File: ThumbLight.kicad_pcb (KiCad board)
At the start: 2 copper layers, 23.5 x 43.8 mm, 6 parts, among them J1 USB_A, U1 DHT11, U2 UA78M33_TO252, U3 ESP-12E, U4 TTL

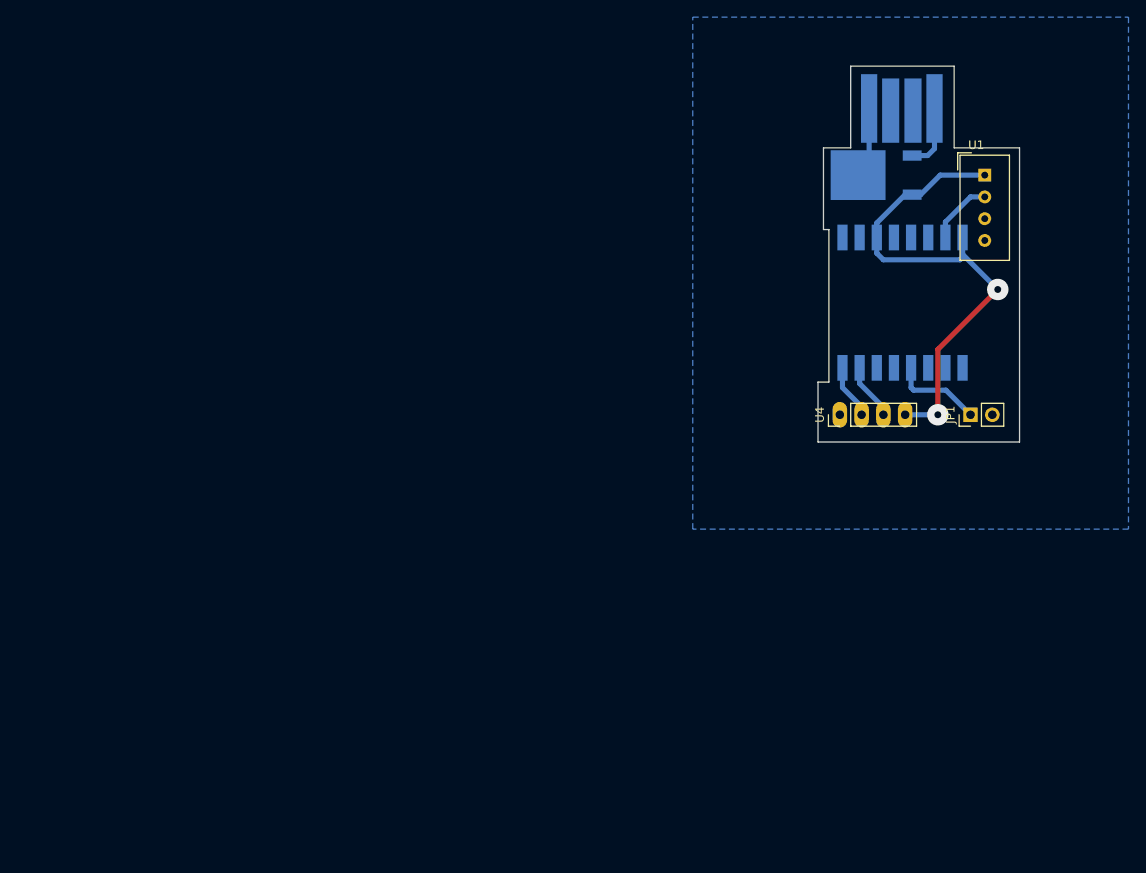
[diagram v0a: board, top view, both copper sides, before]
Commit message: New basic layout
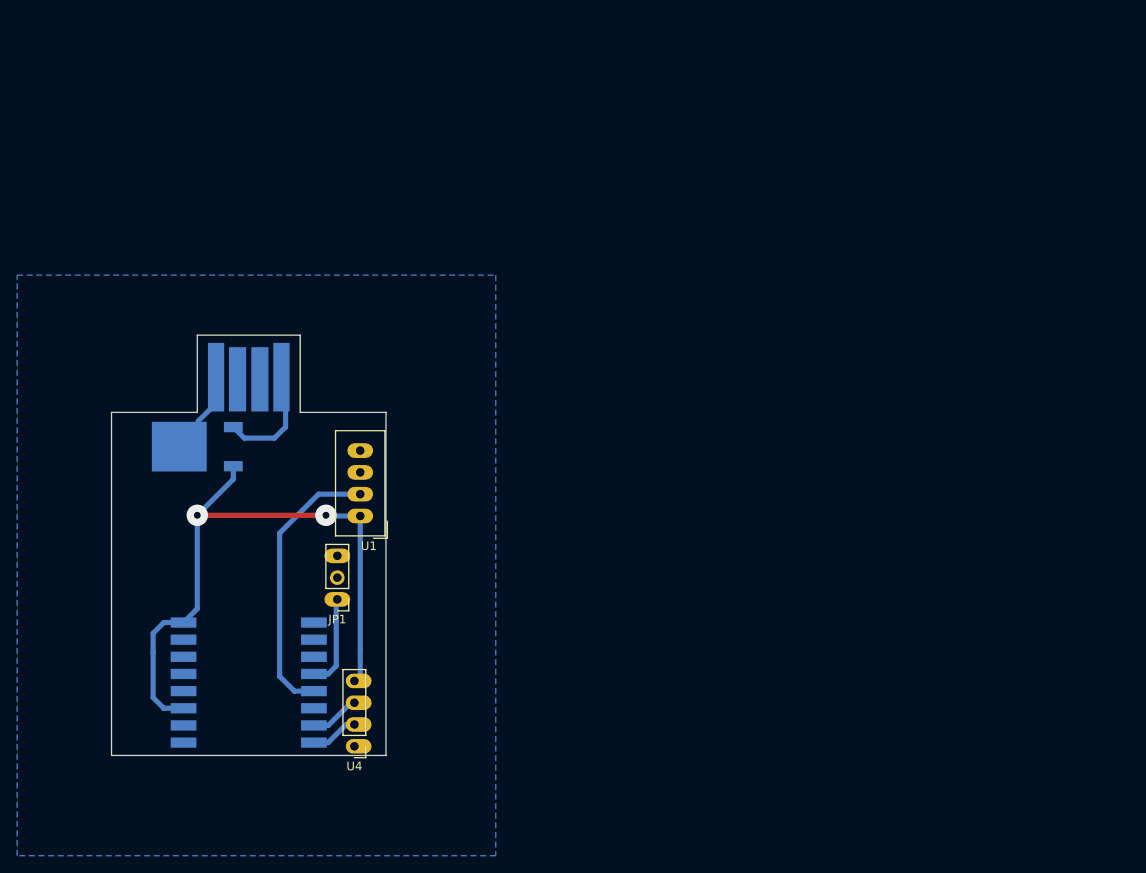
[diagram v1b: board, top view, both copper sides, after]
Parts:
- JP1: footprint Connector_PinHeader_2.54mm:PinHeader_1x02_P2.54mm_Vertical -> Connector_PinHeader_2.54mm:PinHeader_1x03_P2.54mm_Vertical
- moved U3 87.0 mm to (100.0, 116.0), turned to 0 degrees
- moved U2 85.2 mm to (94.0, 85.0)
- moved J1 84.4 mm to (100.0, 72.0)
- moved U1 82.9 mm to (113.0, 93.1), turned to 180 degrees
- moved JP1 76.9 mm to (110.3, 102.8), turned to 180 degrees
- moved U4 68.5 mm to (112.3, 119.9), turned to 180 degrees
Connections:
- U3 pad 19: unconnected-(U3-Pad19) -> TEMP
- U3 pad 7: TEMP -> unconnected-(U3-Pad7)
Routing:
- net TEMP: track 7.78 -> 32.7 mm
- net +3V3: track 60.4 -> 74.8 mm
- net +5V: track 7.63 -> 13.2 mm
- net GND: track 8.30 -> 9.88 mm
- net RX: track 6.61 -> 5.81 mm
- net TX: track 6.39 -> 5.59 mm
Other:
- board size 23.5 x 43.8 mm -> 32 x 49 mm
